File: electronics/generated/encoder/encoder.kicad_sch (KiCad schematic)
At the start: 4 parts, among them J1 CHAIN_3V3_ONLY, U1 AS5048A

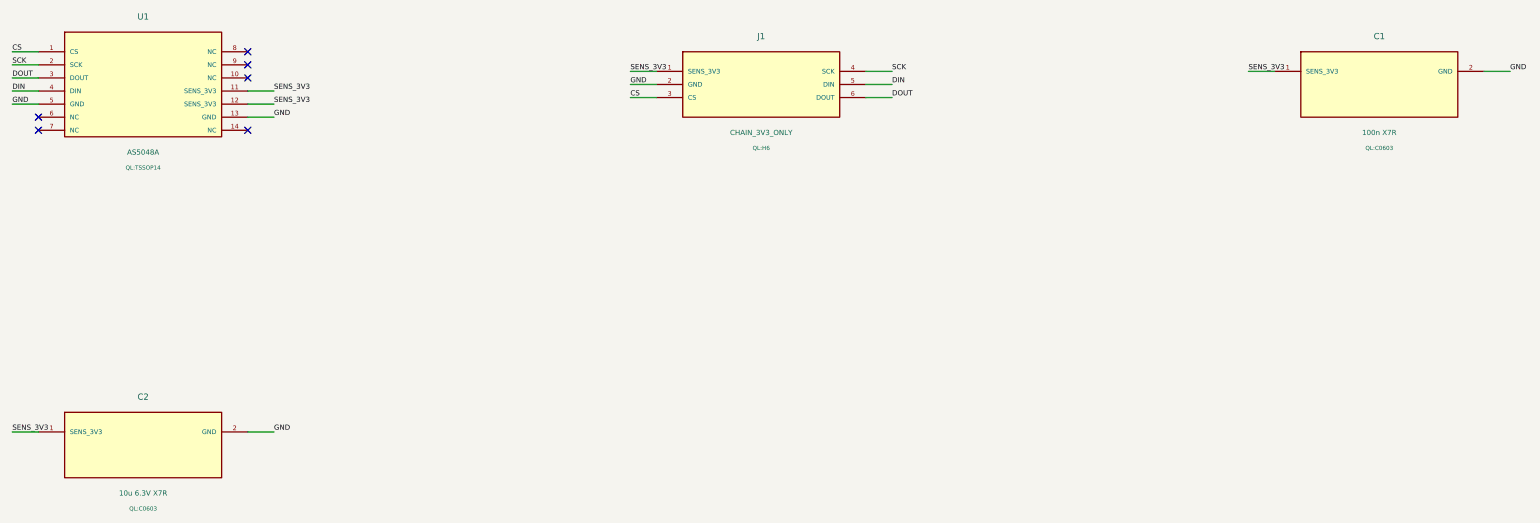
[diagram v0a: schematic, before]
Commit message: build: publish checked electronics/generated [skip ci]
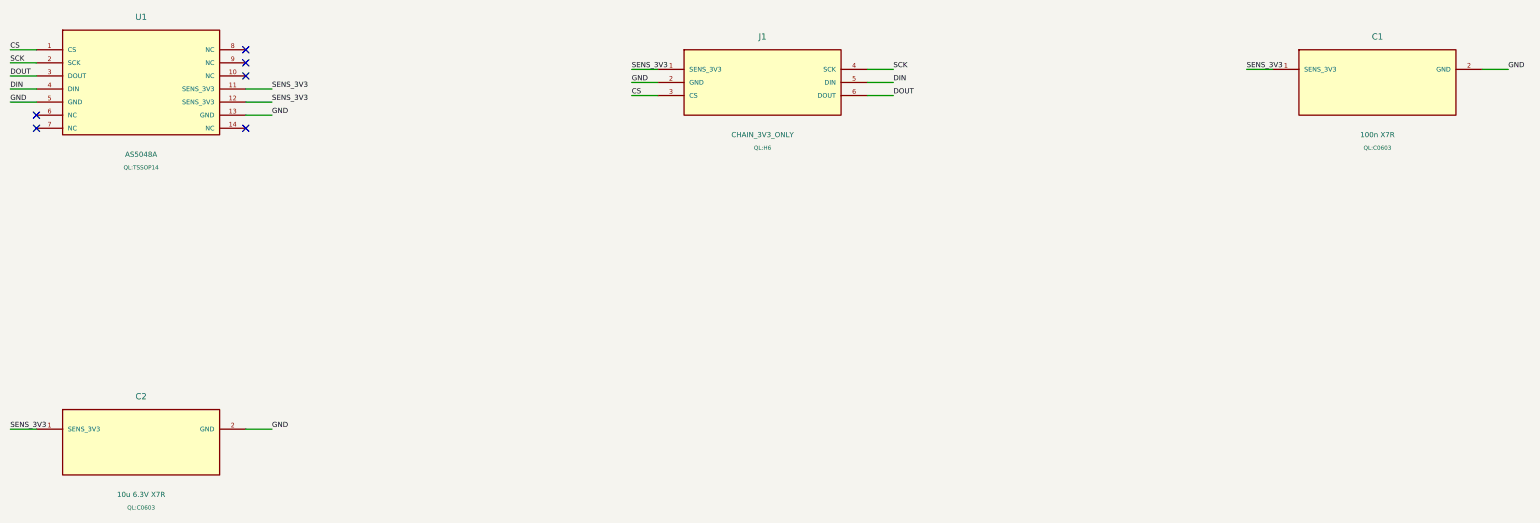
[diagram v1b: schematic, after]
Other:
- moved on the sheet: C1, C2, U1
